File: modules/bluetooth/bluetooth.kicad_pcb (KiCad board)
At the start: 2 copper layers, 24 x 30.5 mm, 2 parts, among them U1 Microchip_BM83

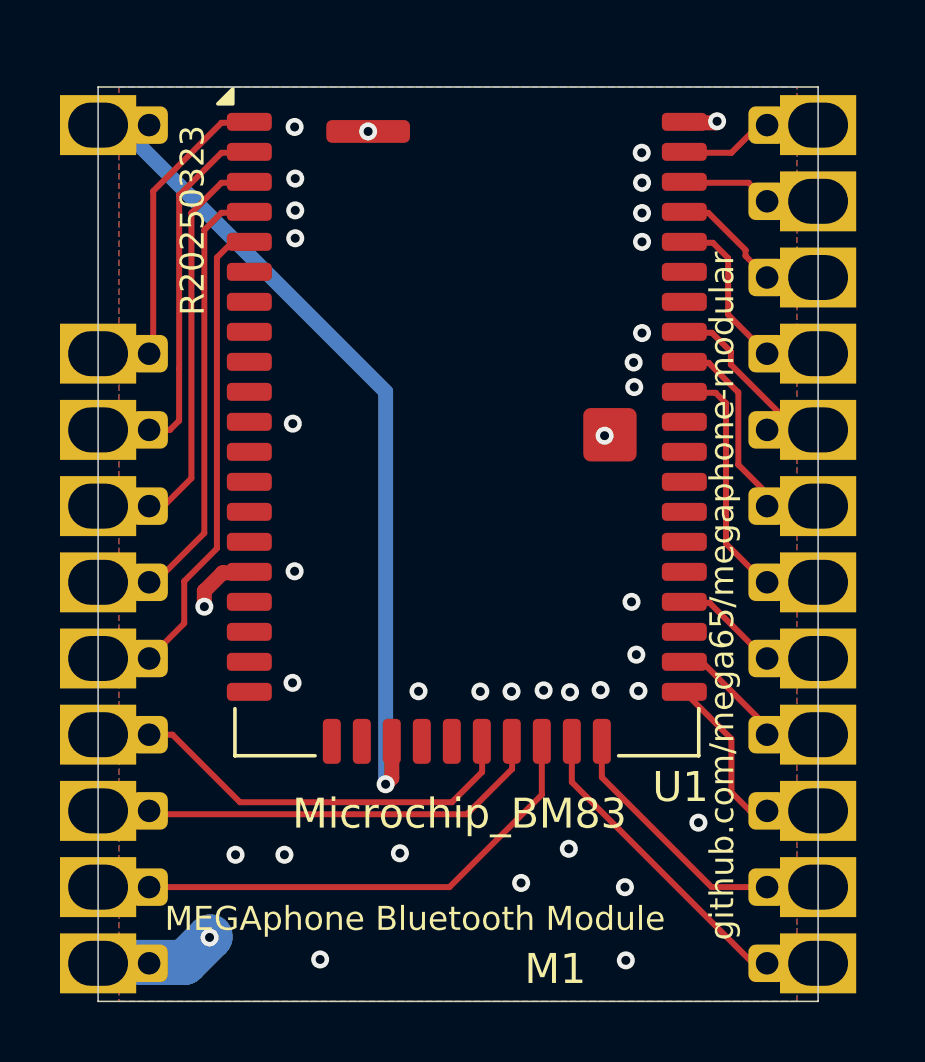
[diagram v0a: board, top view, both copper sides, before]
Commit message: Updating all modules
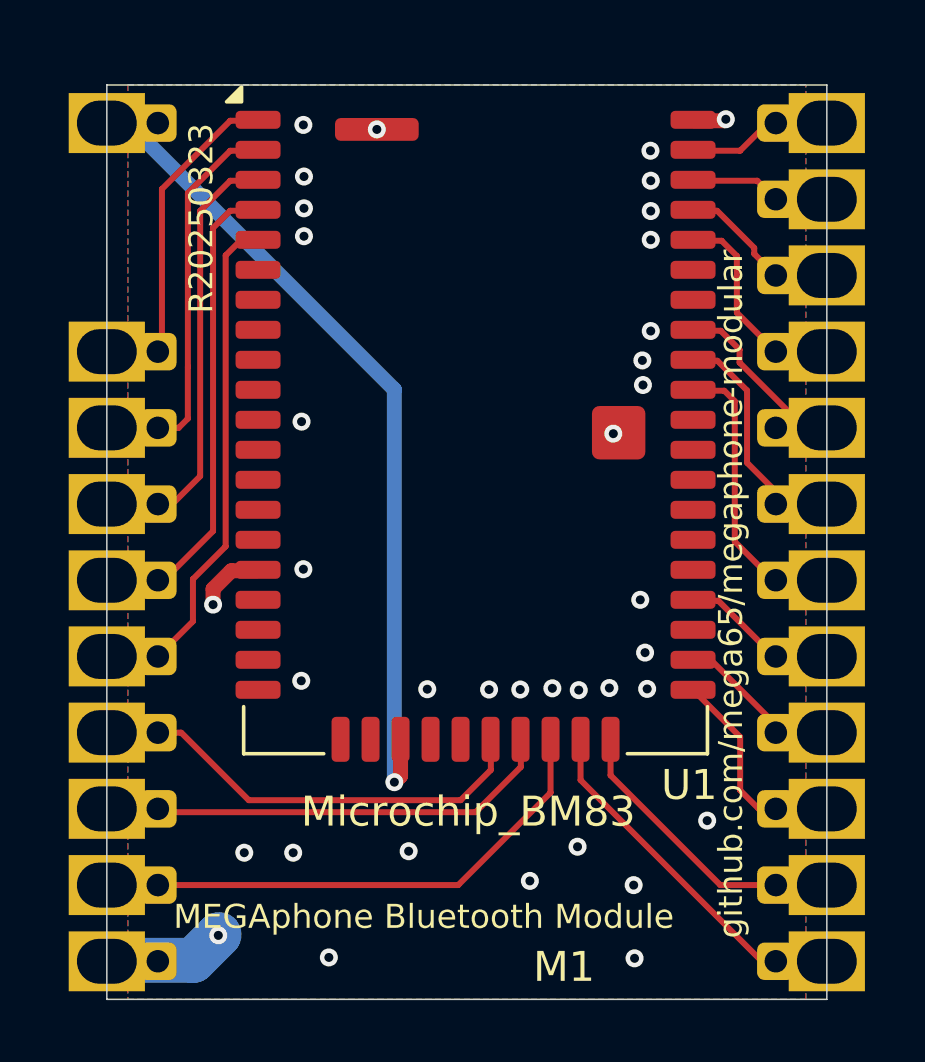
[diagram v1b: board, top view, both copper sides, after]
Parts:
- moved M1 0.30 mm to (109.3, 71.6)
- moved U1 0.30 mm to (109.6, 62.4)
